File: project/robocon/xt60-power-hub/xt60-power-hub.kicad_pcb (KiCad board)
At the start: 2 copper layers, 100 x 25 mm, 13 parts, among them J1 IN, J2 OUT1, J3 OUT2, J4 OUT3, J5 OUT4, J6 OUT5

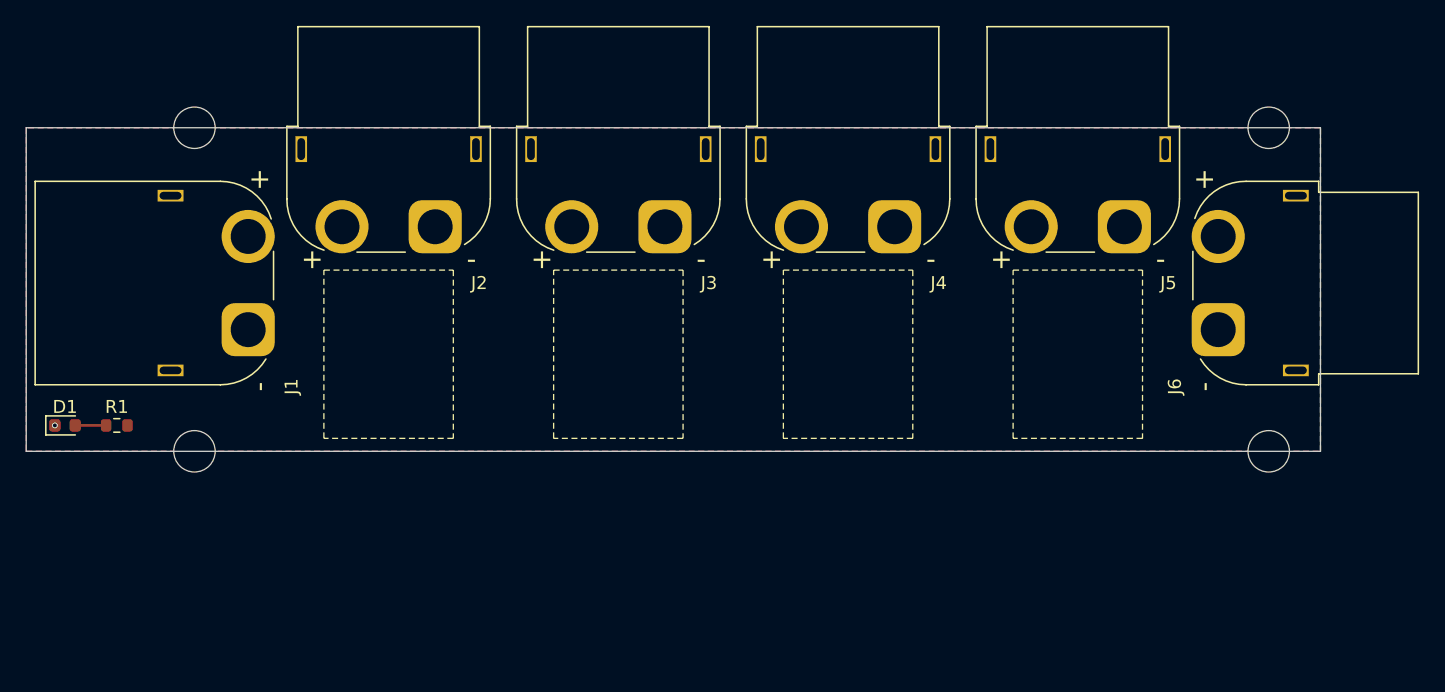
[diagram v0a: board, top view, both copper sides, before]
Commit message: 2026/07/16/09:30
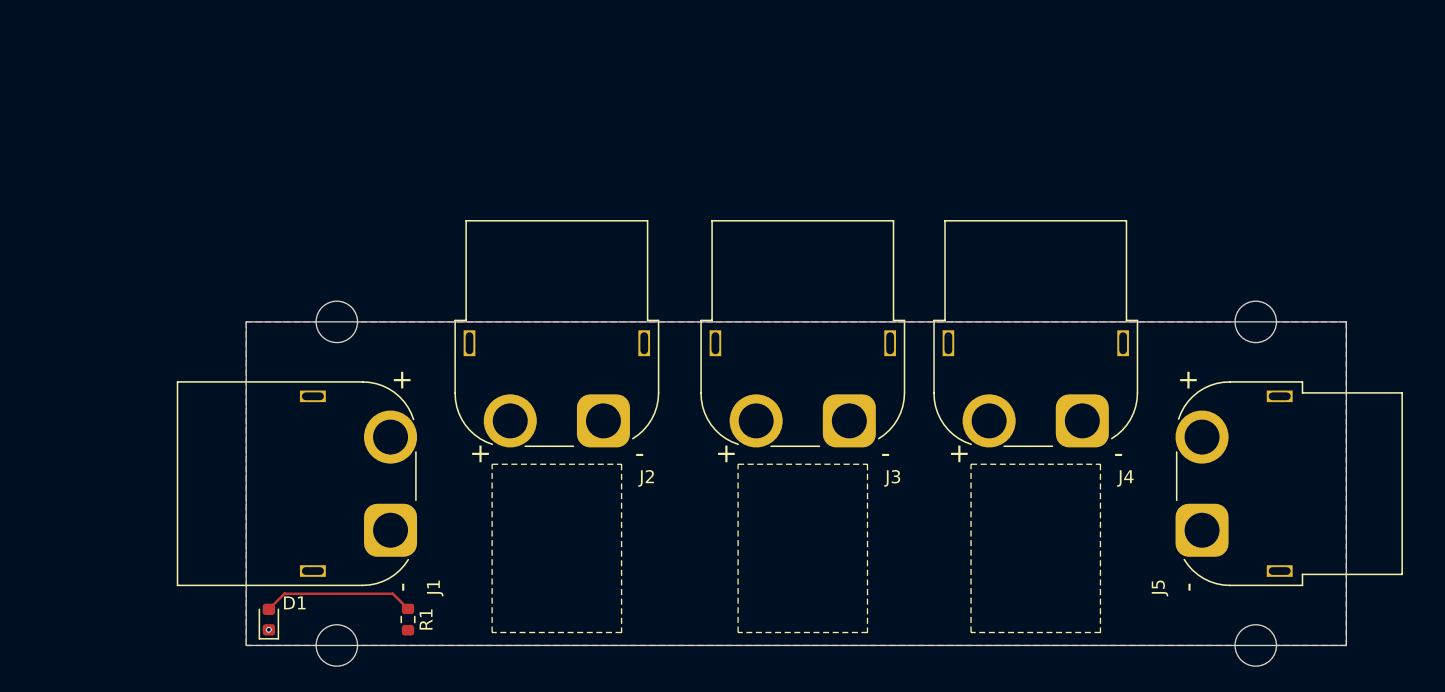
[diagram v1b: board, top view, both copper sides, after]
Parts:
- removed ?: , clipboard:907b6829-476a-4cb7-a632-2a35765c9139
- removed J6: OUT5, Connector_AMASS:AMASS_XT60PW-F_1x02_P7.20mm_Horizontal
- J5: value OUT4 -> OUT5
- moved R1 27.0 mm to (91.5, 107.0), turned to 90 degrees
- moved J5 24.2 mm to (152.8, 100.1), turned to -90 degrees
- moved D1 21.8 mm to (80.8, 107.0), turned to 90 degrees
- moved J4 20.9 mm to (143.6, 91.7)
- moved J3 20.7 mm to (125.6, 91.7)
- moved J2 19.8 mm to (106.6, 91.7)
- moved J1 19.0 mm to (90.2, 100.1)
- moved H1 18.6 mm to (86.0, 84.0)
- moved H2 18.6 mm to (86.0, 109.0)
- moved H3 15.0 mm to (157.0, 109.0)
- moved H4 15.0 mm to (157.0, 84.0)
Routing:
- net Net-(D1-A): track 2.39 -> 11.7 mm
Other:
- board size 100 x 25 mm -> 85 x 25 mm
- board text removed: "基板はいつか燃えるものです。 特にこの基板とその周辺。"
